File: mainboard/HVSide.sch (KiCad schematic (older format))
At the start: 43 parts, among them J10 IMD_TS-, J7 ProminentIndicator, J8 HV, J9 IMD_TS+, Q15 BULB49D, Q16 TSM2312, U13 ISOW7841, U14 Si8900, U15 LTC6259, U16 REF3433, U17 REF2940, U18 FODM611, U19 TPS3700, U20 TCMT1103

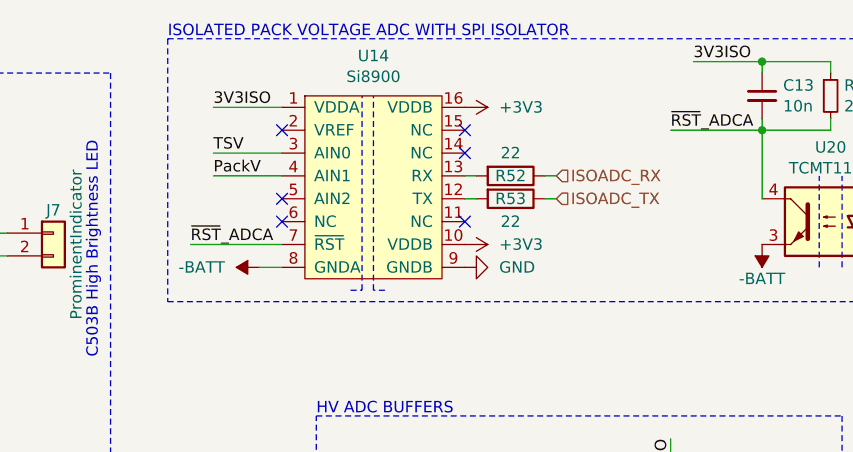
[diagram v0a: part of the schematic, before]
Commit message: i2c isoadc 8901
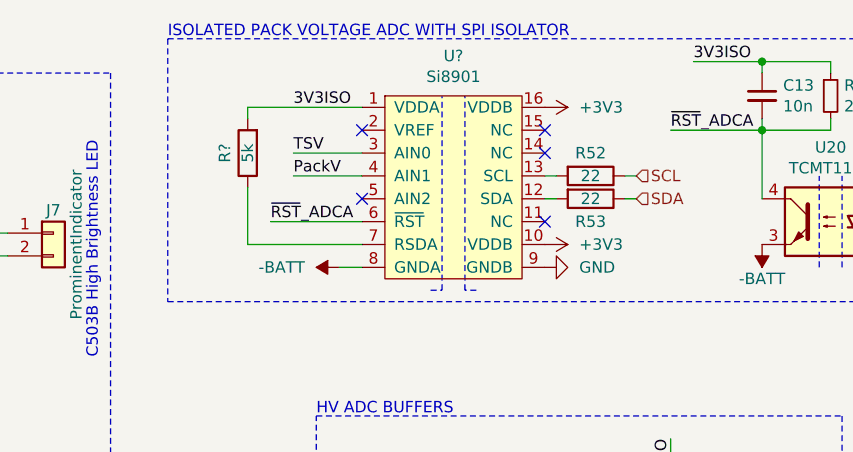
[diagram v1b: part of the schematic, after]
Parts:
- removed U14: Si8900, symbol si8900:Si8900
- added R?: 5k, symbol Device:R
- added U?: Si8901, symbol si8900:Si8901
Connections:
- net +3V3: now also U?.10 (VDDB), U?.16 (VDDB)
- net -BATT: now also U?.8 (GNDA)
- net 3V3ISO: now also R?.2, U?.1 (VDDA)
- net GND: now also U?.9 (GNDB)
- net PackV: now also U?.4 (AIN1)
- net TSV: now also U?.3 (AIN0)
- net ~RST~_ADCA: now also U?.6 (~RST~)
- net at R53.2: now also U?.12 (SDA)
- net at R52.2: now also U?.13 (SCL)
- net ISOADC_RX renamed SCL
- net ISOADC_TX renamed SDA
- new net: R?.1, U?.7 (RSDA)
- no-connect marks 6 -> 5
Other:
- moved on the sheet: R52, R53
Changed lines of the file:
@@
 Wire Notes Line
 	3450 750  3450 1900
-NoConn ~ 4750 1250
-NoConn ~ 4750 1150
+NoConn ~ 5100 1250
+NoConn ~ 5100 1150
 $Comp
 L Device:R R53
 U 1 1 6041ED95
-P 4950 1450
-F 0 "R53" V 4950 1450 50  0000 C CNN
-F 1 "22" V 5050 1450 50  0000 C CNN
-F 2 "" V 4880 1450 50  0001 C CNN
-F 3 "~" H 4950 1450 50  0001 C CNN
-	1    4950 1450
+P 5300 1450
+F 0 "R53" V 5400 1450 50  0000 C CNN
+F 1 "22" V 5300 1450 50  0000 C CNN
+F 2 "" V 5230 1450 50  0001 C CNN
+F 3 "~" H 5300 1450 50  0001 C CNN
+	1    5300 1450
 	0    1    1    0
 $EndComp
@@
 L Device:R R52
 U 1 1 6041E63C
-P 4950 1350
-F 0 "R52" V 4950 1350 50  0000 C CNN
-F 1 "22" V 4850 1350 50  0000 C CNN
-F 2 "" V 4880 1350 50  0001 C CNN
-F 3 "~" H 4950 1350 50  0001 C CNN
-	1    4950 1350
-	0    1    1    0
-$EndComp
-NoConn ~ 3950 1150
-Wire Wire Line
-	3950 1250 3650 1250
-Text Label 3650 1250 0    50   ~ 0
+P 5300 1350
+F 0 "R52" V 5200 1350 50  0000 C CNN
+F 1 "22" V 5300 1350 50  0000 C CNN
+F 2 "" V 5230 1350 50  0001 C CNN
+F 3 "~" H 5300 1350 50  0001 C CNN
+	1    5300 1350
+	0    1    1    0
+$EndComp
+NoConn ~ 4300 1150
+Text Label 4000 1250 0    50   ~ 0
 TSV
-Wire Wire Line
-	3950 1350 3650 1350
-Text Label 3650 1350 0    50   ~ 0
+Text Label 4000 1350 0    50   ~ 0
 PackV
-NoConn ~ 3950 1450
-NoConn ~ 3950 1550
+NoConn ~ 4300 1450
 $Comp
 L power:-BATT #PWR0100
 U 1 1 5B56F926
-P 3850 1750
-F 0 "#PWR0100" H 3850 1600 50  0001 C CNN
-F 1 "-BATT" V 3850 1900 50  0000 L CNN
-F 2 "" H 3850 1750 50  0001 C CNN
-F 3 "" H 3850 1750 50  0001 C CNN
-	1    3850 1750
+P 4200 1750
+F 0 "#PWR0100" H 4200 1600 50  0001 C CNN
+F 1 "-BATT" V 4200 1900 50  0000 L CNN
+F 2 "" H 4200 1750 50  0001 C CNN
+F 3 "" H 4200 1750 50  0001 C CNN
+	1    4200 1750
 	0    -1   -1   0
 $EndComp
-Wire Wire Line
-	3950 1750 3850 1750
-$Comp
-L si8900:Si8900 U14
-U 1 1 603C04CE
-P 4350 1350
-F 0 "U14" H 4350 1875 50  0000 C CNN
-F 1 "Si8900" H 4350 1784 50  0000 C CNN
-F 2 "" H 4200 1800 50  0001 C CNN
-F 3 "" H 4200 1800 50  0001 C CNN
-	1    4350 1350
-	1    0    0    -1
-$EndComp
-Wire Wire Line
-	3650 1050 3950 1050
-Text Label 3650 1050 0    50   ~ 0
+Text Label 4000 1050 0    50   ~ 0
 3V3ISO
 Text Notes 3450 750  0    50   ~ 0
 ISOLATED PACK VOLTAGE ADC WITH SPI ISOLATOR
-NoConn ~ 4750 1550
+NoConn ~ 5100 1550
 $Comp
 L power:+3V3 #PWR015
 U 1 1 6046C081
-P 4750 1050
-F 0 "#PWR015" H 4750 900 50  0001 C CNN
-F 1 "+3V3" V 4750 1200 50  0000 L CNN
-F 2 "" H 4750 1050 50  0001 C CNN
-F 3 "" H 4750 1050 50  0001 C CNN
-	1    4750 1050
+P 5100 1050
+F 0 "#PWR015" H 5100 900 50  0001 C CNN
+F 1 "+3V3" V 5100 1200 50  0000 L CNN
+F 2 "" H 5100 1050 50  0001 C CNN
+F 3 "" H 5100 1050 50  0001 C CNN
+	1    5100 1050
 	0    1    1    0
 $EndComp
@@
 L power:+3V3 #PWR099
 U 1 1 6046CB1E
-P 4750 1650
-F 0 "#PWR099" H 4750 1500 50  0001 C CNN
-F 1 "+3V3" V 4750 1800 50  0000 L CNN
-F 2 "" H 4750 1650 50  0001 C CNN
-F 3 "" H 4750 1650 50  0001 C CNN
-	1    4750 1650
+P 5100 1650
+F 0 "#PWR099" H 5100 1500 50  0001 C CNN
+F 1 "+3V3" V 5100 1800 50  0000 L CNN
+F 2 "" H 5100 1650 50  0001 C CNN
+F 3 "" H 5100 1650 50  0001 C CNN
+	1    5100 1650
 	0    1    1    0
 $EndComp
@@
 L power:GND #PWR0143
 U 1 1 6046D345
-P 4750 1750
-F 0 "#PWR0143" H 4750 1500 50  0001 C CNN
-F 1 "GND" V 4750 1600 50  0000 R CNN
-F 2 "" H 4750 1750 50  0001 C CNN
-F 3 "" H 4750 1750 50  0001 C CNN
-	1    4750 1750
+P 5100 1750
+F 0 "#PWR0143" H 5100 1500 50  0001 C CNN
+F 1 "GND" V 5100 1600 50  0000 R CNN
+F 2 "" H 5100 1750 50  0001 C CNN
+F 3 "" H 5100 1750 50  0001 C CNN
+	1    5100 1750
 	0    -1   -1   0
 $EndComp
 Wire Wire Line
-	4800 1350 4750 1350
-Wire Wire Line
-	4750 1450 4800 1450
-Wire Wire Line
-	5100 1350 5150 1350
-Wire Wire Line
-	5150 1450 5100 1450
-Text HLabel 5150 1450 2    50   Input ~ 0
-ISOADC_TX
-Text HLabel 5150 1350 2    50   Input ~ 0
-ISOADC_RX
-Text Label 3550 1650 0    50   ~ 0
+	5150 1350 5100 1350
+Wire Wire Line
+	5100 1450 5150 1450
+Wire Wire Line
+	5450 1350 5500 1350
+Wire Wire Line
+	5500 1450 5450 1450
+Text HLabel 5500 1450 2    50   Input ~ 0
+SDA
+Text HLabel 5500 1350 2    50   Input ~ 0
+SCL
+Text Label 3900 1550 0    50   ~ 0
 ~RST~_ADCA
-Wire Wire Line
-	3550 1650 3950 1650
 Text Label 5650 1150 0    50   ~ 0
 ~RST~_ADCA
@@
 $EndComp
 Wire Notes Line
-	4250 1850 4300 1850
-Wire Notes Line
-	4300 1850 4300 1000
-Wire Notes Line
-	4400 1850 4350 1850
-Wire Notes Line
-	4350 1850 4350 1000
+	4600 1850 4650 1850
+Wire Notes Line
+	4650 1850 4650 1000
+Wire Notes Line
+	4800 1850 4750 1850
+Wire Notes Line
+	4750 1850 4750 1000
 Wire Notes Line
 	6400 1750 6400 1350
@@
 Wire Wire Line
 	6050 1150 6050 1450
+Wire Wire Line
+	4300 1750 4200 1750
+Wire Wire Line
+	4300 1350 4000 1350
+Wire Wire Line
+	4300 1250 4000 1250
+$Comp
+L si8900:Si8901 U?
+U 1 1 603E5D4E
+P 4700 1350
+F 0 "U?" H 4700 1875 50  0000 C CNN
+F 1 "Si8901" H 4700 1784 50  0000 C CNN
+F 2 "" H 4550 1800 50  0001 C CNN
+F 3 "" H 4550 1800 50  0001 C CNN
+	1    4700 1350
+	1    0    0    -1
+$EndComp
+$Comp
+L Device:R R?
+U 1 1 603F9D47
+P 3800 1250
+F 0 "R?" V 3900 1250 50  0000 C CNN
+F 1 "5k" V 3800 1250 50  0000 C CNN
+F 2 "" V 3730 1250 50  0001 C CNN
+F 3 "~" H 3800 1250 50  0001 C CNN
+	1    3800 1250
+	-1   0    0    1
+$EndComp
+Wire Wire Line
+	3900 1550 4300 1550
+Wire Wire Line
+	3800 1650 3800 1400
+Wire Wire Line
+	3800 1050 3800 1100
+Wire Wire Line
+	3800 1650 4300 1650
+Wire Wire Line
+	3800 1050 4300 1050
 $EndSCHEMATC
